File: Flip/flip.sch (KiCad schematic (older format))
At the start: 18 parts, among them J1 CHANNEL, J2 COILS, J3 IDC1, J4 GROUND, J5 IDC2, Q1 Q_NPN_BEC, Q2 Q_NPN_BEC, Q3 Q_NPN_BEC, Q4 Q_NPN_BEC

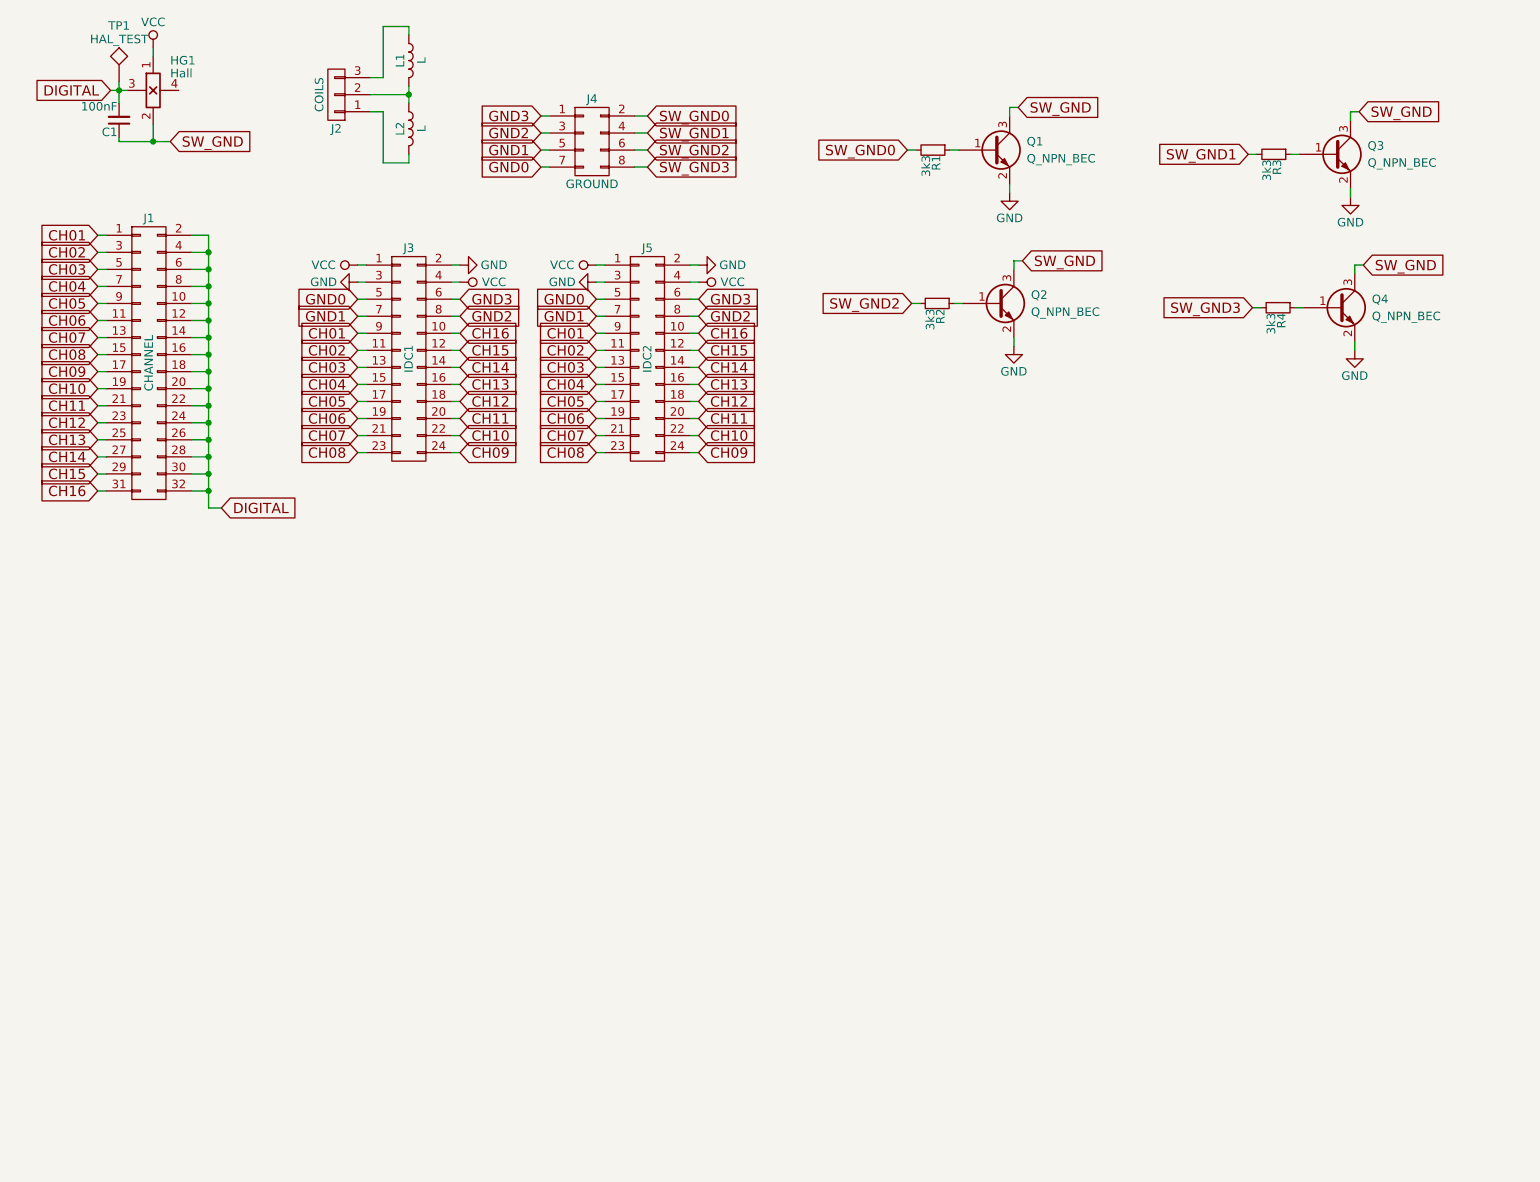
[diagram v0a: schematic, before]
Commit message: new PCB WIP
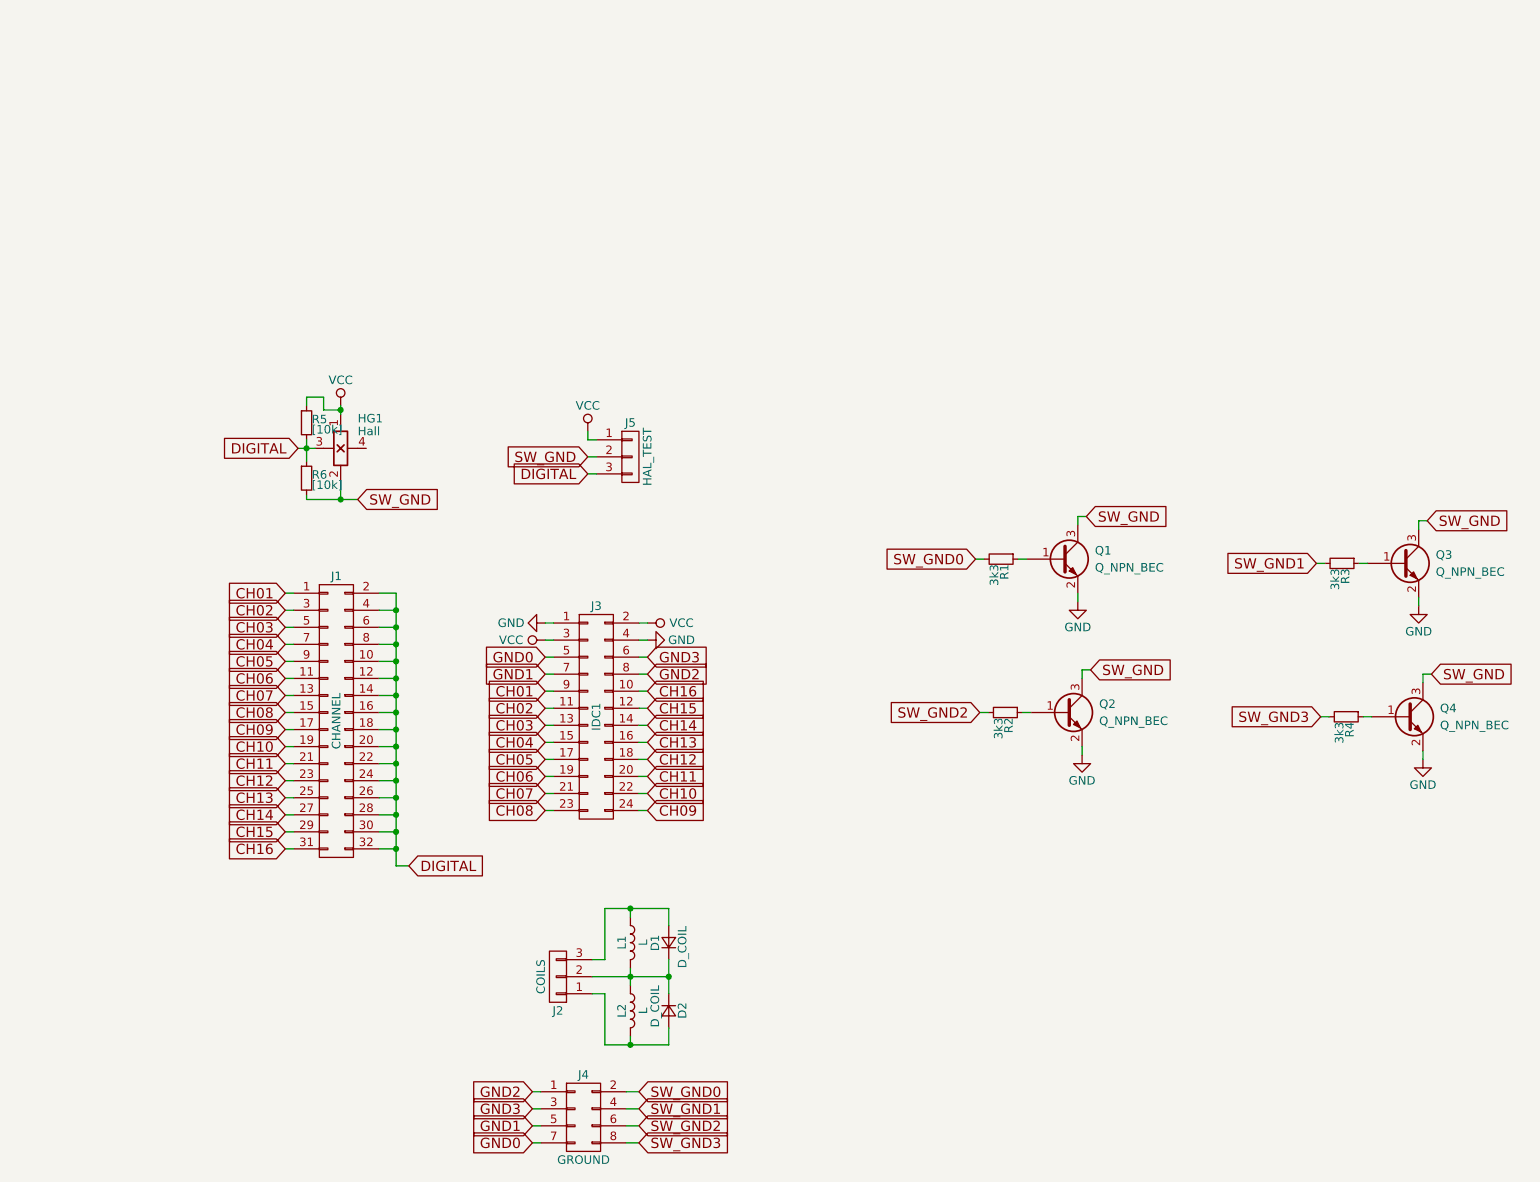
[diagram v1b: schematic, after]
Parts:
- removed C1: 100nF, Capacitors_SMD:C_0805_HandSoldering, symbol C_Small
- removed J5: IDC2, Pin_Headers:Pin_Header_Straight_2x12_Pitch2.54mm, symbol CONN_02X12
- removed TP1: HAL_TEST, Pin_Headers:Pin_Header_Straight_1x01_Pitch2.54mm, symbol TEST
- added D1, D2: D_COIL, Diodes_SMD:D_0805, symbol D_Small
- added J5: HAL_TEST, Pin_Headers:Pin_Header_Straight_1x03_Pitch2.54mm, symbol CONN_01X03
- added R5, R6: [10k], Resistors_SMD:R_0603_HandSoldering, symbol R_Small
- J3: footprint Pin_Headers:Pin_Header_Straight_2x12_Pitch2.54mm -> #MOJABIBLIOTEKA:IDC_edge
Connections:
- net DIGITAL: now also J5.3 (P3), R5.2, R6.1
- net GND: now also J3.1 (P1), J3.4 (P4); no longer J3.2 (P2), J3.3 (P3)
- net GND2: now also J4.1 (P1); no longer J4.3 (P3)
- net GND3: now also J4.3 (P3); no longer J4.1 (P1)
- net SW_GND: now also J5.2 (P2), R6.2
- net VCC: now also J3.2 (P2), J3.3 (P3), J5.1 (P1), R5.1; no longer J3.1 (P1), J3.4 (P4)
- net at J2.2 (P2), L1.2, L2.1: now also D1.1 (K), D2.1 (K)
- net at J2.1 (P1), L2.2: now also D2.2 (A)
- net at J2.3 (P3), L1.1: now also D1.2 (A)
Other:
- moved on the sheet: HG1, J1, J2, J3, J4, L1, L2, Q1, Q2, Q3, Q4, R1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
